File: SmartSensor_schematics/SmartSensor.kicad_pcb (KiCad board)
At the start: 4 copper layers, 79.2 x 74.4 mm, 54 parts, among them IC1 DS1337+, IC2 SHT31-DIS-B, IC3 VEML7700-TT, J6 Barrel_Jack, J8 6 PIN ISP, Q1 MMBF170, Q2 MMBF170, Q3 MMBF170, Q4 MMBF170, Q5 MMBF170, SW1 SW_Push, U1 AZ1117-3.3, U2 MCP9808_MSOP, U3 DMG2301l, U4 ATmega328P-AU, U5 XBee_SMT, U6 MCP1640BCH, X1 XTAL

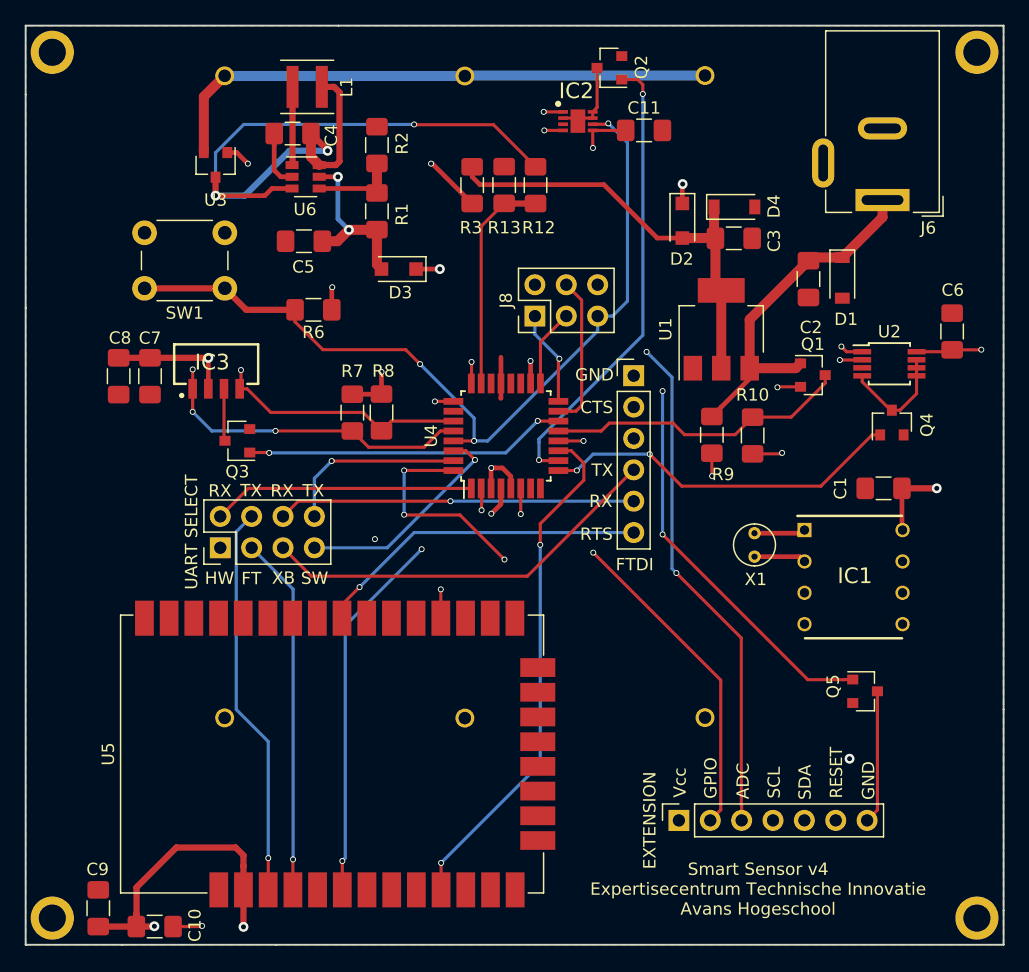
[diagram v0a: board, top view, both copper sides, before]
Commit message: hardware: update hardware
Update the smart sensor hardware.

Signed-off-by: Michel Megens <michel@michelmegens.net>
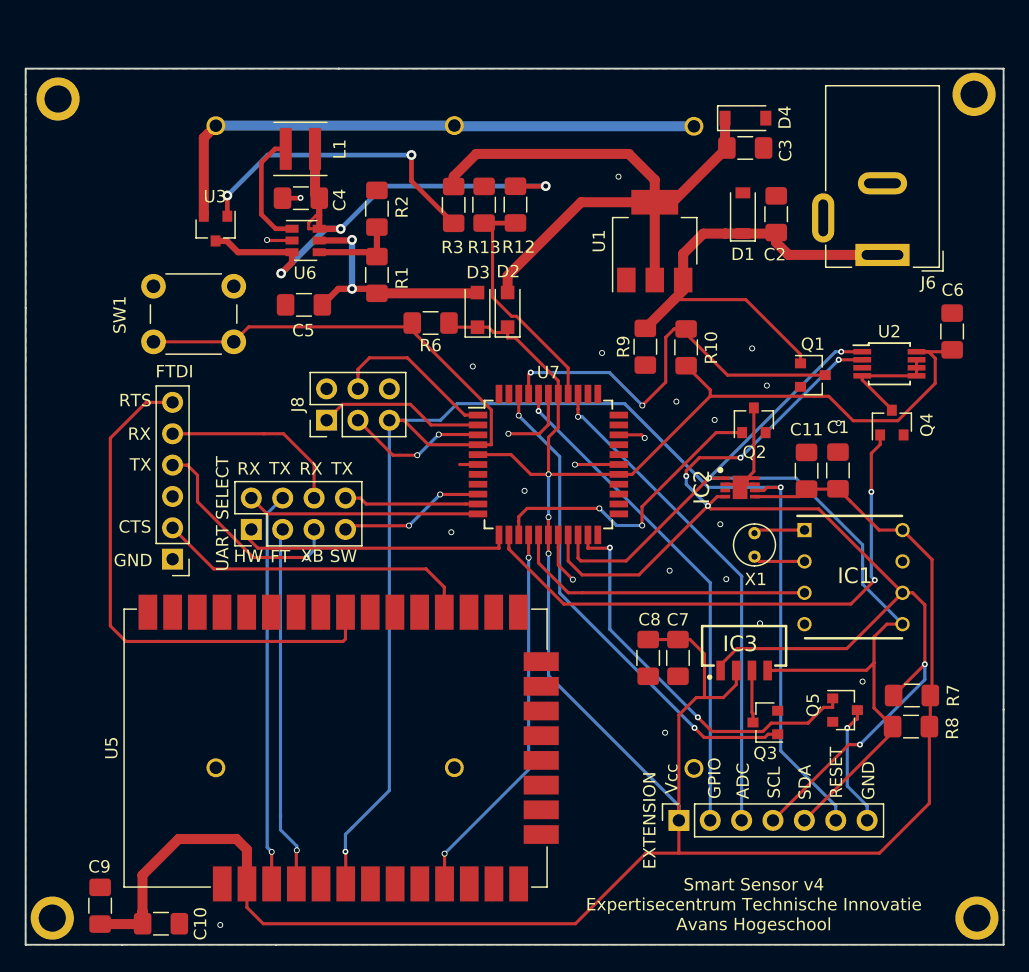
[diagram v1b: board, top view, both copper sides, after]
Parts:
- removed U4: ATmega328P-AU, Package_QFP:TQFP-32_7x7mm_P0.8mm
- added U7: ATmega1284P-AU, Package_QFP:TQFP-44_10x10mm_P0.8mm, F.Cu at (118.6, 119.4)
- moved R7 50.8 mm to (148.0, 138.1), turned to 180 degrees
- moved R8 49.9 mm to (148.0, 140.6), turned to 180 degrees
- moved C8 48.6 mm to (126.7, 135.0)
- moved IC3 48.5 mm to (131.0, 135.6)
- moved Q3 48.5 mm to (136.2, 140.2)
- moved C7 48.5 mm to (129.1, 135.0)
- moved FTDI 40.2 mm to (88.2, 127.0), turned to 180 degrees
- moved IC2 32.4 mm to (134.1, 121.2)
- moved Q2 30.8 mm to (135.2, 115.8), turned to 90 degrees
- moved C11 30.5 mm to (139.5, 119.9), turned to 90 degrees
- moved J8 18.9 mm to (100.6, 115.8)
- moved D2 15.9 mm to (115.3, 106.8), turned to 90 degrees
- moved D1 9.60 mm to (134.3, 99.0), turned to 90 degrees
- moved R6 9.54 mm to (109.1, 107.9)
- moved R10 8.94 mm to (129.7, 109.9)
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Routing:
- net +3V3: track 67.4 -> 249.6 mm, vias 14 -> 3
- net SDA: track 134.9 -> 86.0 mm, vias 3 -> 2
- net SCL: track 142.0 -> 104.6 mm, vias 5 -> 6
- net EXT_ENABLE: track 52.2 -> 32.5 mm, vias 3 -> 2
- net +BATT: track 64.0 -> 46.3 mm
- net INTA_IO2: track 42.6 -> 24.9 mm, vias 3 -> 0
- net ADC1: track 57.6 -> 40.3 mm, vias 3 -> 1
- net LDO_out: track 35.9 -> 52.8 mm
- net TMP_IO5: track 29.4 -> 45.6 mm
- net XBEE_RTS: track 27.1 -> 43.3 mm, vias 1 -> 0
- net FTDI_TX: track 32.9 -> 17.7 mm, vias 0 -> 1
- net APDS_IO9: track 26.1 -> 40.1 mm
- net FTDI_RX: track 28.9 -> 15.2 mm, vias 1 -> 0
- net SHT31_IO6: track 37.3 -> 24.4 mm
- net XB_SLEEP: track 41.8 -> 31.1 mm
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- removed copper zone on PWR.Cu, net +3V3
- removed copper zone on Util.Cu, net GND
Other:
- board size 79.2 x 74.4 mm -> 79.2 x 70.9 mm
- copper layers 4 -> 2
- net class Default: trace_width 0.25 -> 0.254; via_dia 0.8 -> 0.4826; via_drill 0.4 -> 0.3302
